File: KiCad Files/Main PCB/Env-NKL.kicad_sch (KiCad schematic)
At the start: 244 parts, among them J1 TYPE-C-31-M-14, J2 Conn_01x03_Male, SW1 EVQP7C, SW2 EVQP7C, U1 W25Q16J, U2 3.3V SOT-23-5 5.5V 3.3V, U3 RP2040, Y1 3225_4P 12MHz

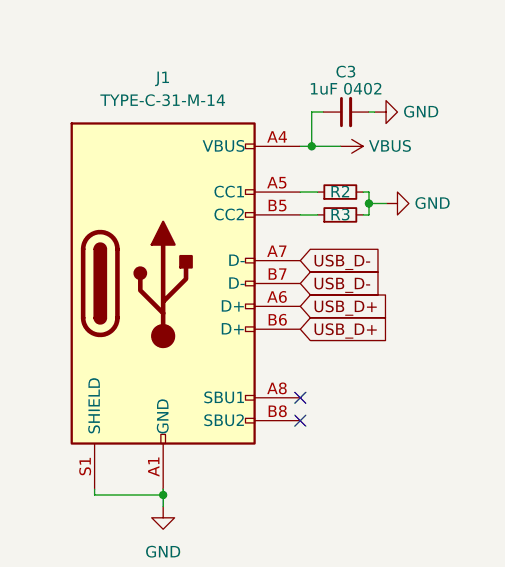
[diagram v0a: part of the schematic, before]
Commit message: experimenting & some curiosities with KiCad 7
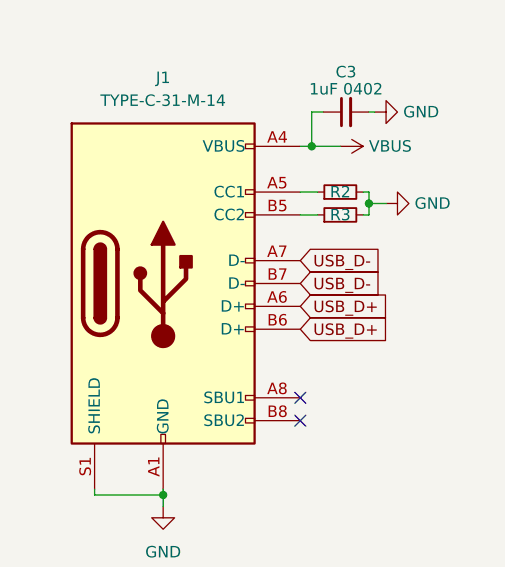
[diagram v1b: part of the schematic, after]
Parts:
- U1: footprint Package_SO:SOIC-8_3.9x4.9mm_P1.27mm -> Package_SON:SON-8-1EP_3x2mm_P0.5mm_EP1.4x1.6mm
